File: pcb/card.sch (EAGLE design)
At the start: 19 parts, among them IC1 74HC14D, IC2 W25X32, Q1 2N7002

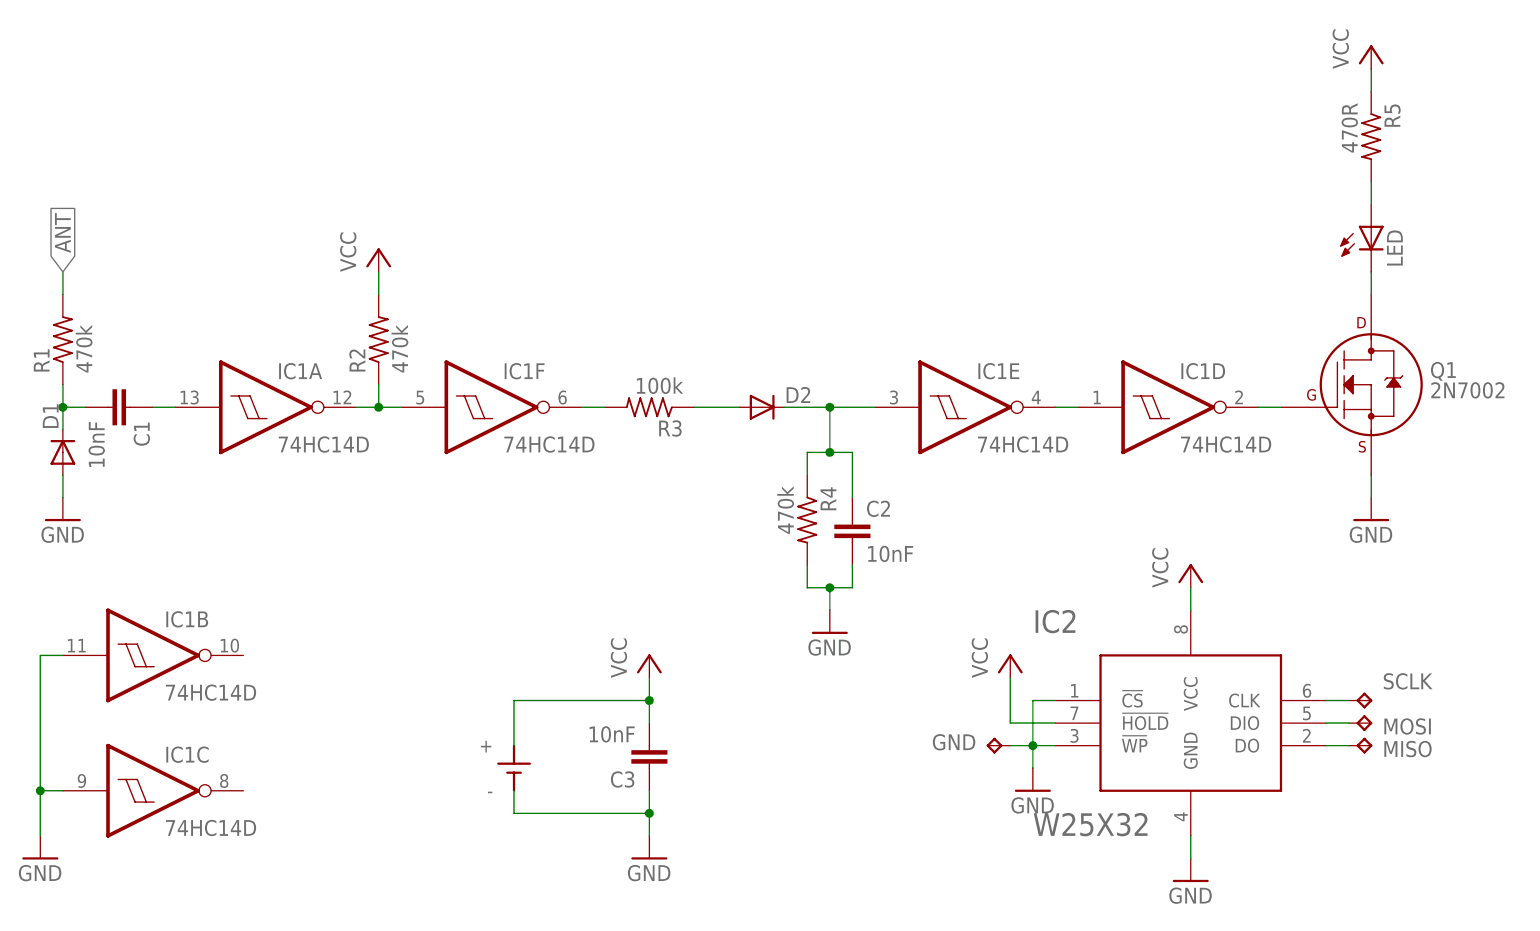
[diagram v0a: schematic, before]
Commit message: Compacted & improved the design.
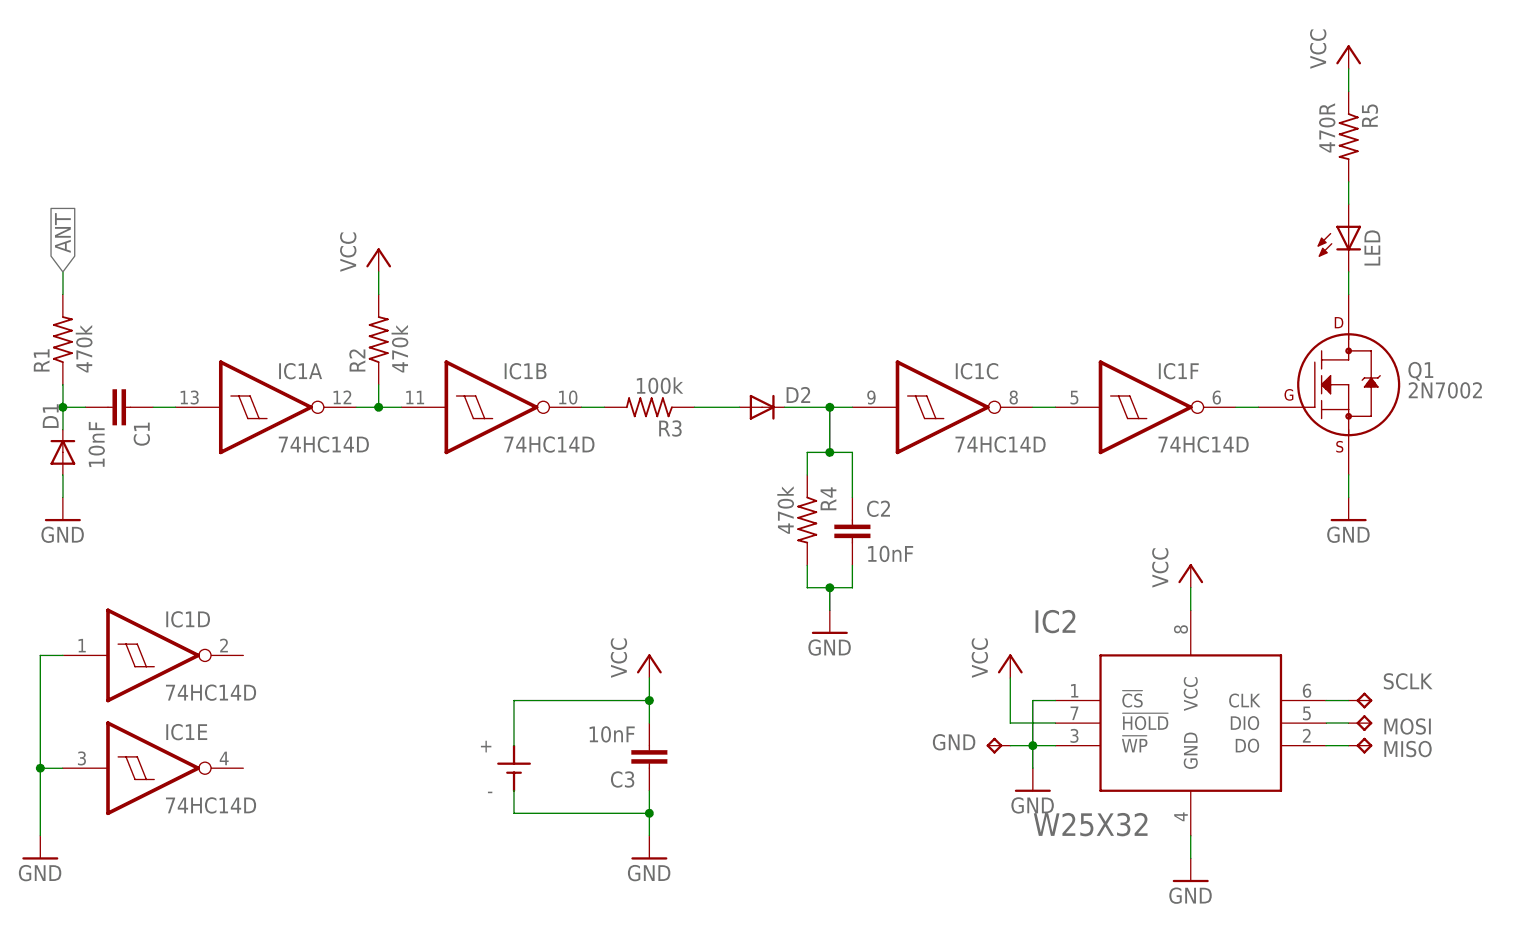
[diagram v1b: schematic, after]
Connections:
- net GND: now also IC1D.I, IC1E.I; no longer IC1B.I, IC1C.I
- net N$11: now also IC1C.O, IC1F.I; no longer IC1D.I, IC1E.O
- net N$12: now also IC1F.O; no longer IC1D.O
- net N$5: now also IC1B.I; no longer IC1F.I
- net N$6: now also IC1B.O; no longer IC1F.O
- net N$8: now also IC1C.I; no longer IC1E.I
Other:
- moved on the sheet: IC1B, IC1C, IC1D, IC1E, IC1F, LED, Q1, R5
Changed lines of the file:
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@@
 <instance part="P+1" gate="VCC" x="60.96" y="22.86"/>
 <instance part="P+2" gate="VCC" x="30.48" y="68.58"/>
-<instance part="P+3" gate="VCC" x="142.24" y="91.44"/>
+<instance part="P+3" gate="VCC" x="139.7" y="91.44"/>
 <instance part="R1" gate="G$1" x="-5.08" y="58.42" rot="R90"/>
 <instance part="R3" gate="G$1" x="60.96" y="50.8" rot="R180"/>
@@
 <instance part="GND3" gate="1" x="-7.62" y="0"/>
 <instance part="GND4" gate="1" x="81.28" y="25.4"/>
-<instance part="GND5" gate="1" x="142.24" y="38.1"/>
+<instance part="GND5" gate="1" x="139.7" y="38.1"/>
 <instance part="IC1" gate="A" x="17.78" y="50.8"/>
-<instance part="IC1" gate="B" x="5.08" y="22.86"/>
-<instance part="IC1" gate="C" x="5.08" y="7.62"/>
-<instance part="IC1" gate="D" x="119.38" y="50.8"/>
-<instance part="IC1" gate="E" x="96.52" y="50.8"/>
-<instance part="IC1" gate="F" x="43.18" y="50.8"/>
+<instance part="IC1" gate="B" x="43.18" y="50.8"/>
+<instance part="IC1" gate="C" x="93.98" y="50.8"/>
+<instance part="IC1" gate="D" x="5.08" y="22.86"/>
+<instance part="IC1" gate="E" x="5.08" y="10.16"/>
+<instance part="IC1" gate="F" x="116.84" y="50.8"/>
 <instance part="D2" gate="G$1" x="73.66" y="50.8"/>
-<instance part="LED" gate="G$1" x="142.24" y="71.12"/>
+<instance part="LED" gate="G$1" x="139.7" y="71.12"/>
 <instance part="R2" gate="G$1" x="30.48" y="58.42" rot="R90"/>
 <instance part="C3" gate="G$1" x="60.96" y="10.16" rot="R180"/>
@@
 </instance>
 <instance part="D1" gate="G$1" x="-5.08" y="45.72" rot="R90"/>
-<instance part="R5" gate="G$1" x="142.24" y="81.28" rot="R270"/>
-<instance part="Q1" gate="G$1" x="142.24" y="53.34"/>
+<instance part="R5" gate="G$1" x="139.7" y="81.28" rot="R270"/>
+<instance part="Q1" gate="G$1" x="139.7" y="53.34"/>
 </instances>
 <busses>
@@
 <net name="GND" class="0">
 <segment>
-<pinref part="IC1" gate="B" pin="I"/>
 <pinref part="GND3" gate="1" pin="GND"/>
-<wire x1="-5.08" y1="22.86" x2="-7.62" y2="22.86" width="0.1524" layer="91"/>
-<wire x1="-7.62" y1="22.86" x2="-7.62" y2="7.62" width="0.1524" layer="91"/>
-<pinref part="IC1" gate="C" pin="I"/>
-<wire x1="-7.62" y1="7.62" x2="-7.62" y2="2.54" width="0.1524" layer="91"/>
-<wire x1="-5.08" y1="7.62" x2="-7.62" y2="7.62" width="0.1524" layer="91"/>
-<junction x="-7.62" y="7.62"/>
+<wire x1="-7.62" y1="22.86" x2="-7.62" y2="10.16" width="0.1524" layer="91"/>
+<wire x1="-7.62" y1="10.16" x2="-7.62" y2="2.54" width="0.1524" layer="91"/>
+<pinref part="IC1" gate="E" pin="I"/>
+<wire x1="-5.08" y1="10.16" x2="-7.62" y2="10.16" width="0.1524" layer="91"/>
+<junction x="-7.62" y="10.16"/>
+<pinref part="IC1" gate="D" pin="I"/>
+<wire x1="-7.62" y1="22.86" x2="-5.08" y2="22.86" width="0.1524" layer="91"/>
 </segment>
 <segment>
@@
 <segment>
 <pinref part="GND5" gate="1" pin="GND"/>
-<wire x1="142.24" y1="43.18" x2="142.24" y2="40.64" width="0.1524" layer="91"/>
+<wire x1="139.7" y1="43.18" x2="139.7" y2="40.64" width="0.1524" layer="91"/>
 <pinref part="Q1" gate="G$1" pin="S"/>
 </segment>
@@
 <net name="N$5" class="0">
 <segment>
-<pinref part="IC1" gate="F" pin="I"/>
 <pinref part="R2" gate="G$1" pin="1"/>
-<wire x1="30.48" y1="50.8" x2="33.02" y2="50.8" width="0.1524" layer="91"/>
 <wire x1="30.48" y1="53.34" x2="30.48" y2="50.8" width="0.1524" layer="91"/>
 <pinref part="IC1" gate="A" pin="O"/>
 <wire x1="30.48" y1="50.8" x2="27.94" y2="50.8" width="0.1524" layer="91"/>
+<pinref part="IC1" gate="B" pin="I"/>
+<wire x1="33.02" y1="50.8" x2="30.48" y2="50.8" width="0.1524" layer="91"/>
 <junction x="30.48" y="50.8"/>
 </segment>
@@
 <pinref part="R5" gate="G$1" pin="1"/>
 <pinref part="P+3" gate="VCC" pin="VCC"/>
-<wire x1="142.24" y1="88.9" x2="142.24" y2="86.36" width="0.1524" layer="91"/>
-</segment>
-</net>
-<net name="N$6" class="0">
-<segment>
-<pinref part="IC1" gate="F" pin="O"/>
-<pinref part="R3" gate="G$1" pin="2"/>
-<wire x1="53.34" y1="50.8" x2="55.88" y2="50.8" width="0.1524" layer="91"/>
+<wire x1="139.7" y1="88.9" x2="139.7" y2="86.36" width="0.1524" layer="91"/>
 </segment>
 </net>
@@
 <segment>
 <pinref part="D2" gate="G$1" pin="C"/>
-<pinref part="IC1" gate="E" pin="I"/>
 <wire x1="76.2" y1="50.8" x2="81.28" y2="50.8" width="0.1524" layer="91"/>
-<wire x1="86.36" y1="50.8" x2="81.28" y2="50.8" width="0.1524" layer="91"/>
 <wire x1="81.28" y1="50.8" x2="81.28" y2="45.72" width="0.1524" layer="91"/>
 <pinref part="R4" gate="G$1" pin="1"/>
@@
 <wire x1="83.82" y1="45.72" x2="83.82" y2="40.64" width="0.1524" layer="91"/>
 <junction x="81.28" y="45.72"/>
+<pinref part="IC1" gate="C" pin="I"/>
+<wire x1="83.82" y1="50.8" x2="81.28" y2="50.8" width="0.1524" layer="91"/>
 <junction x="81.28" y="50.8"/>
-</segment>
-</net>
-<net name="N$11" class="0">
-<segment>
-<pinref part="IC1" gate="E" pin="O"/>
-<pinref part="IC1" gate="D" pin="I"/>
-<wire x1="106.68" y1="50.8" x2="109.22" y2="50.8" width="0.1524" layer="91"/>
-</segment>
-</net>
-<net name="N$12" class="0">
-<segment>
-<pinref part="IC1" gate="D" pin="O"/>
-<wire x1="129.54" y1="50.8" x2="132.08" y2="50.8" width="0.1524" layer="91"/>
-<pinref part="Q1" gate="G$1" pin="G"/>
 </segment>
 </net>
@@
 <pinref part="LED" gate="G$1" pin="A"/>
 <pinref part="R5" gate="G$1" pin="2"/>
-<wire x1="142.24" y1="76.2" x2="142.24" y2="73.66" width="0.1524" layer="91"/>
+<wire x1="139.7" y1="76.2" x2="139.7" y2="73.66" width="0.1524" layer="91"/>
 </segment>
 </net>
@@
 <segment>
 <pinref part="LED" gate="G$1" pin="C"/>
-<wire x1="142.24" y1="66.04" x2="142.24" y2="63.5" width="0.1524" layer="91"/>
+<wire x1="139.7" y1="66.04" x2="139.7" y2="63.5" width="0.1524" layer="91"/>
 <pinref part="Q1" gate="G$1" pin="D"/>
 </segment>
 </net>
+<net name="N$12" class="0">
+<segment>
+<pinref part="Q1" gate="G$1" pin="G"/>
+<pinref part="IC1" gate="F" pin="O"/>
+<wire x1="127" y1="50.8" x2="129.54" y2="50.8" width="0.1524" layer="91"/>
+</segment>
+</net>
+<net name="N$6" class="0">
+<segment>
+<pinref part="R3" gate="G$1" pin="2"/>
+<pinref part="IC1" gate="B" pin="O"/>
+<wire x1="53.34" y1="50.8" x2="55.88" y2="50.8" width="0.1524" layer="91"/>
+</segment>
+</net>
+<net name="N$11" class="0">
+<segment>
+<pinref part="IC1" gate="F" pin="I"/>
+<pinref part="IC1" gate="C" pin="O"/>
+<wire x1="104.14" y1="50.8" x2="106.68" y2="50.8" width="0.1524" layer="91"/>
+</segment>
+</net>
